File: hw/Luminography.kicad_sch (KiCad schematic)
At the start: 109 parts, among them J1 USB_C_Receptacle_PowerOnly_6P, J2 Conn_01x04, Q1 MMBT3904, Q2 2N7002, SW1 SW_Push, U1 LTC4054ES5-4.2, U10 MAX98357AETE+, U100 BH1750FVI-TR, U101 BH1750FVI-TR, U102 BH1750FVI-TR, U103 BH1750FVI-TR, U104 BH1750FVI-TR, U105 BH1750FVI-TR, U106 BH1750FVI-TR, U107 BH1750FVI-TR, U108 BH1750FVI-TR, U109 BH1750FVI-TR, U110 BH1750FVI-TR, U111 BH1750FVI-TR, U112 BH1750FVI-TR, U113 BH1750FVI-TR, U114 BH1750FVI-TR, U115 BH1750FVI-TR, U116 BH1750FVI-TR, U117 BH1750FVI-TR, U118 BH1750FVI-TR, U119 BH1750FVI-TR, U120 BH1750FVI-TR, U121 BH1750FVI-TR, U122 BH1750FVI-TR, U123 BH1750FVI-TR, U2 XS3A1T3157GMX, U3 SPX3819M5-L-3-3, U4 MAX17048G+T10, U5 STM32G030K6Tx, U6 ZJY128R-IG01, U7 W25Q16JVUXIQ, U8 BMI270, U9 MMC5603NJ, X1 12.288MHz

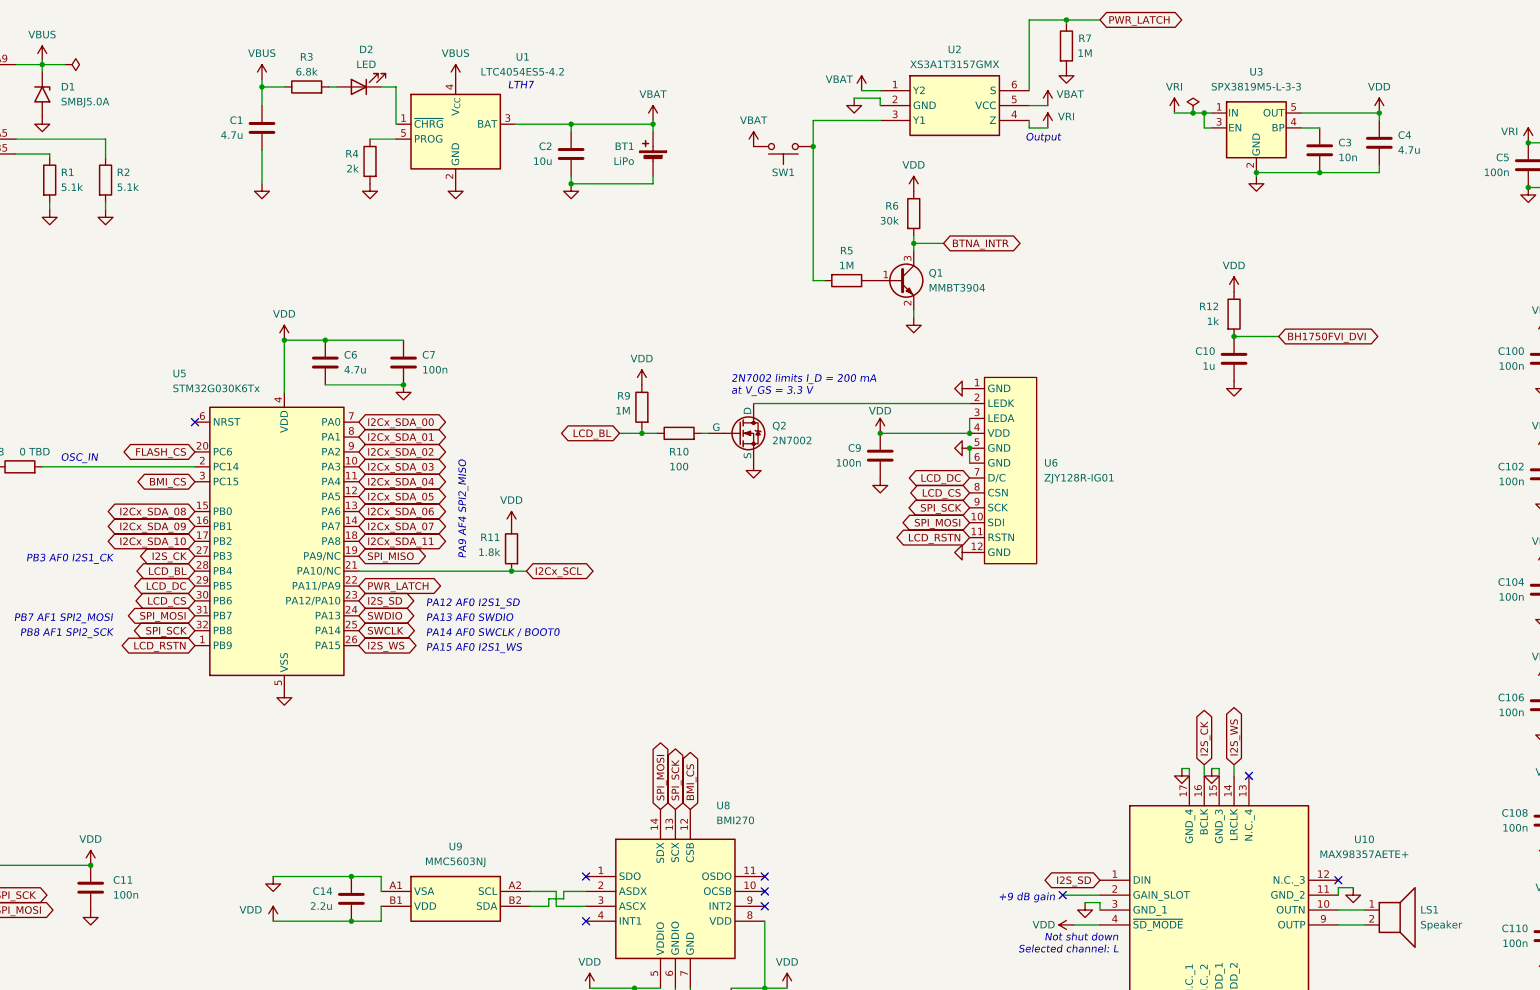
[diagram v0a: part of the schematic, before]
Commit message: 🚧 Routing WIP
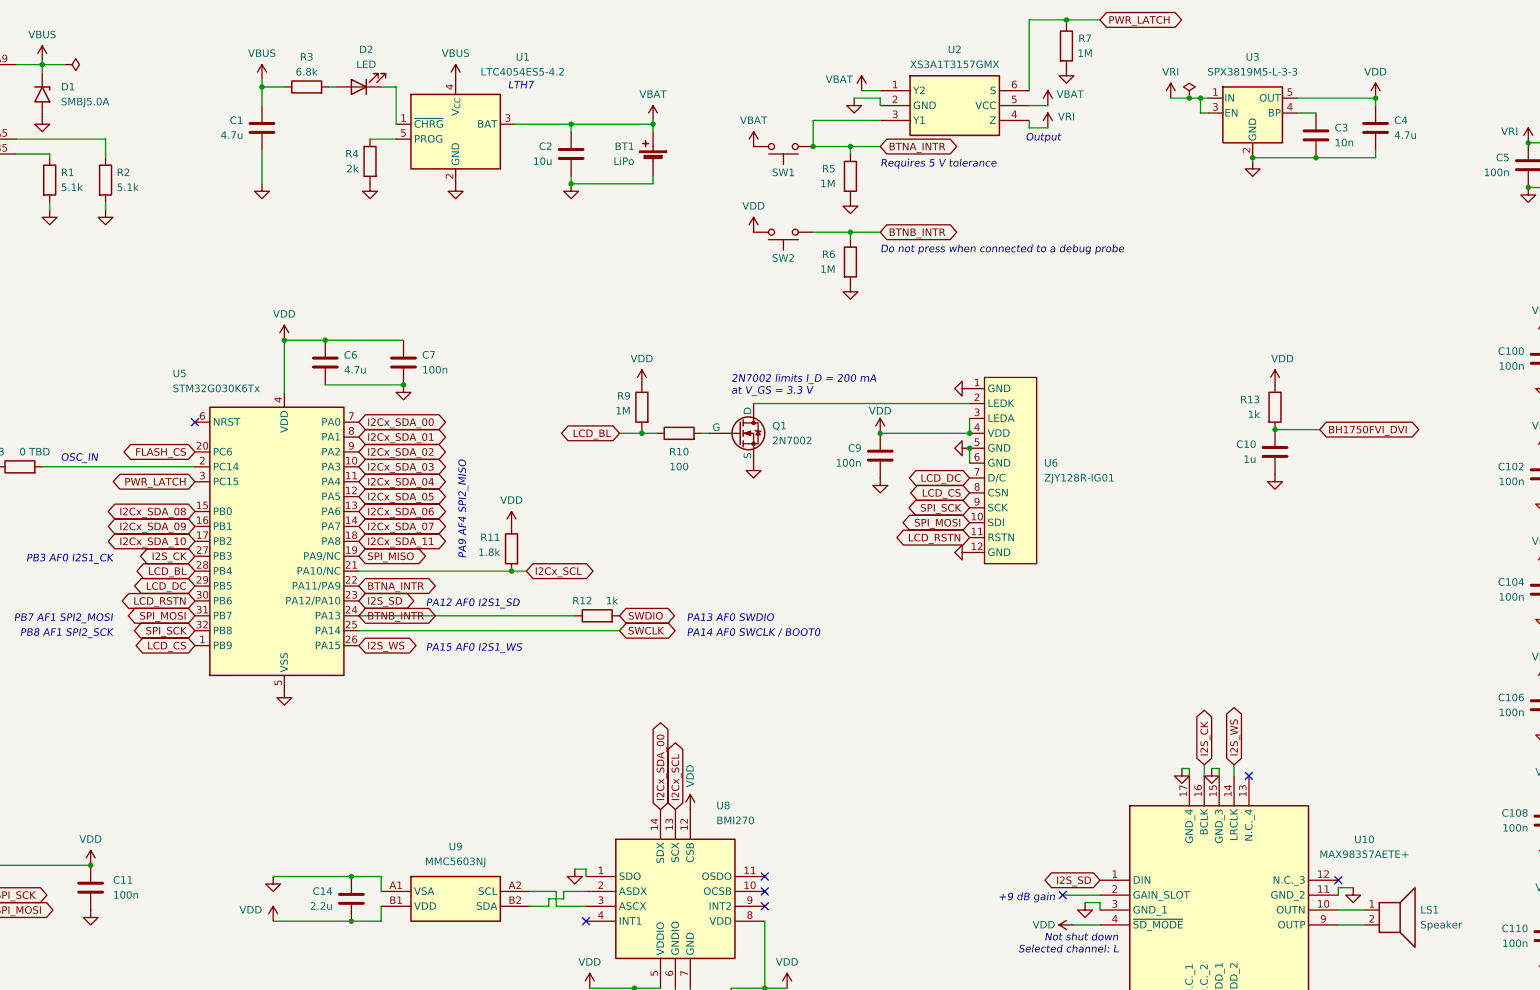
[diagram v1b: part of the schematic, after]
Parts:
- removed Q1: MMBT3904, Package_TO_SOT_SMD:SOT-23, symbol Transistor_BJT:MMBT3904
- removed R5: 1M, Resistor_SMD:R_0402_1005Metric, symbol Device:R
- added R12: 1k, Resistor_SMD:R_0402_1005Metric, symbol Device:R
- added R6: 1M, Resistor_SMD:R_0402_1005Metric, symbol Device:R
- added SW2: SW_Push, Button_Switch_SMD:SW_SPST_TL3342, symbol Switch:SW_Push
- R5: renamed from R6; value 30k -> 1M
- renumbered Q2 to Q1, R12 to R13
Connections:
- net BTNA_INTR: now also R5.1, SW1.2, U2.3 (Y1), U5.22 (PA11/PA9); no longer R5.2
- net GND: now also R5.2, U8.1 (SDO), R6.2
- net I2Cx_SCL: now also U8.13 (SCX)
- net I2Cx_SDA_00: now also U8.14 (SDX)
- net LCD_CS: now also U5.1 (PB9); no longer U5.30 (PB6)
- net LCD_RSTN: now also U5.30 (PB6); no longer U5.1 (PB9)
- net PWR_LATCH: now also U5.3 (PC15); no longer U5.22 (PA11/PA9)
- net SPI_MOSI: no longer U8.14 (SDX)
- net SPI_SCK: no longer U8.13 (SCX)
- net SWDIO: now also R12.2; no longer U5.24 (PA13)
- net VDD: now also U8.12 (CSB), SW2.1; no longer R5.1
- removed net BMI_CS: U5.3 (PC15), U8.12 (CSB)
- new net BTNB_INTR: R12.1, R6.1, SW2.2, U5.24 (PA13)
- no-connect marks 16 -> 15
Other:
- note added: "Do not press when connected to a debug probe"
- note added: "Requires 5 V tolerance"
- moved on the sheet: C10, C3, C4, R13, R5, U3

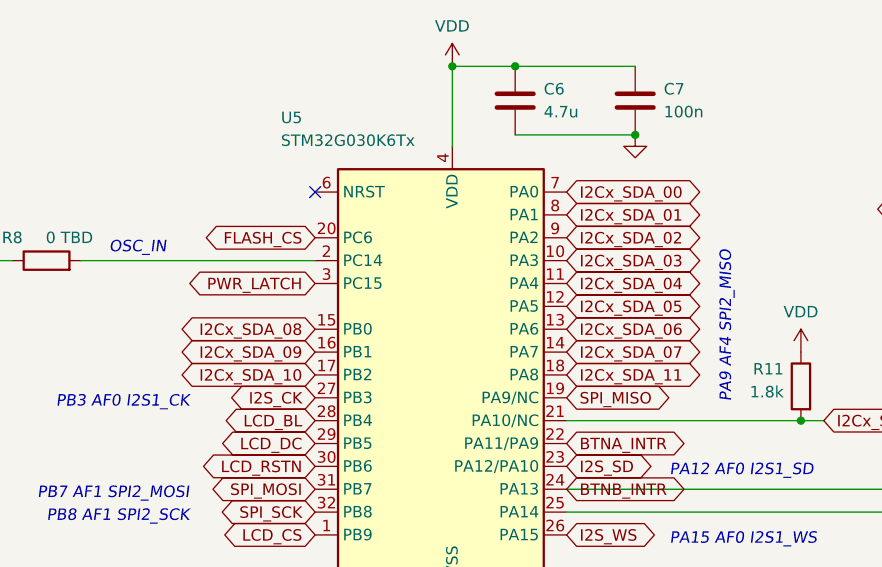
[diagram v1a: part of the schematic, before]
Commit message: Board design almost done, do later
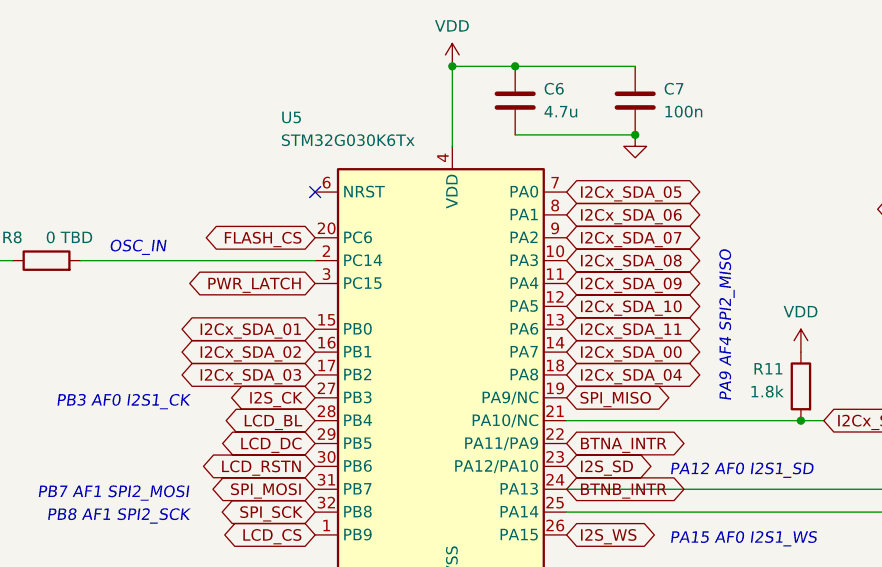
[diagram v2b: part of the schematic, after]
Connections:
- net I2Cx_SDA_00: now also U5.14 (PA7); no longer U5.7 (PA0)
- net I2Cx_SDA_01: now also U5.15 (PB0); no longer U5.8 (PA1)
- net I2Cx_SDA_02: now also U5.16 (PB1); no longer U5.9 (PA2)
- net I2Cx_SDA_03: now also U5.17 (PB2); no longer U5.10 (PA3)
- net I2Cx_SDA_04: now also U5.18 (PA8); no longer U5.11 (PA4)
- net I2Cx_SDA_05: now also U5.7 (PA0); no longer U5.12 (PA5)
- net I2Cx_SDA_06: now also U5.8 (PA1); no longer U5.13 (PA6)
- net I2Cx_SDA_07: now also U5.9 (PA2); no longer U5.14 (PA7)
- net I2Cx_SDA_08: now also U5.10 (PA3); no longer U5.15 (PB0)
- net I2Cx_SDA_09: now also U5.11 (PA4); no longer U5.16 (PB1)
- net I2Cx_SDA_10: now also U5.12 (PA5); no longer U5.17 (PB2)
- net I2Cx_SDA_11: now also U5.13 (PA6); no longer U5.18 (PA8)
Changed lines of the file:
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@@
     )
   )
-  (global_label "I2Cx_SDA_02" (shape bidirectional) (at 100.33 88.9 0) (fields_autoplaced)
+  (global_label "I2Cx_SDA_07" (shape bidirectional) (at 100.33 88.9 0) (fields_autoplaced)
     (effects (font (size 1.27 1.27)) (justify left))
     (property "Intersheetrefs" "${INTERSHEET_REFS}" (at 116.4612 88.9 0)
@@
     )
   )
-  (global_label "I2Cx_SDA_07" (shape bidirectional) (at 100.33 101.6 0) (fields_autoplaced)
+  (global_label "I2Cx_SDA_00" (shape bidirectional) (at 100.33 101.6 0) (fields_autoplaced)
     (effects (font (size 1.27 1.27)) (justify left))
     (property "Intersheetrefs" "${INTERSHEET_REFS}" (at 116.4612 101.6 0)
@@
     )
   )
-  (global_label "I2Cx_SDA_03" (shape bidirectional) (at 100.33 91.44 0) (fields_autoplaced)
+  (global_label "I2Cx_SDA_08" (shape bidirectional) (at 100.33 91.44 0) (fields_autoplaced)
     (effects (font (size 1.27 1.27)) (justify left))
     (property "Intersheetrefs" "${INTERSHEET_REFS}" (at 116.4612 91.44 0)
@@
     )
   )
-  (global_label "I2Cx_SDA_08" (shape bidirectional) (at 72.39 99.06 180) (fields_autoplaced)
+  (global_label "I2Cx_SDA_01" (shape bidirectional) (at 72.39 99.06 180) (fields_autoplaced)
     (effects (font (size 1.27 1.27)) (justify right))
     (property "Intersheetrefs" "${INTERSHEET_REFS}" (at 56.2588 99.06 0)
@@
     )
   )
-  (global_label "I2Cx_SDA_10" (shape bidirectional) (at 72.39 104.14 180) (fields_autoplaced)
+  (global_label "I2Cx_SDA_03" (shape bidirectional) (at 72.39 104.14 180) (fields_autoplaced)
     (effects (font (size 1.27 1.27)) (justify right))
     (property "Intersheetrefs" "${INTERSHEET_REFS}" (at 56.2588 104.14 0)
@@
     )
   )
-  (global_label "I2Cx_SDA_04" (shape bidirectional) (at 100.33 93.98 0) (fields_autoplaced)
+  (global_label "I2Cx_SDA_09" (shape bidirectional) (at 100.33 93.98 0) (fields_autoplaced)
     (effects (font (size 1.27 1.27)) (justify left))
     (property "Intersheetrefs" "${INTERSHEET_REFS}" (at 116.4612 93.98 0)
@@
     )
   )
-  (global_label "I2Cx_SDA_01" (shape bidirectional) (at 100.33 86.36 0) (fields_autoplaced)
+  (global_label "I2Cx_SDA_06" (shape bidirectional) (at 100.33 86.36 0) (fields_autoplaced)
     (effects (font (size 1.27 1.27)) (justify left))
     (property "Intersheetrefs" "${INTERSHEET_REFS}" (at 116.4612 86.36 0)
@@
     )
   )
-  (global_label "I2Cx_SDA_11" (shape bidirectional) (at 100.33 104.14 0) (fields_autoplaced)
+  (global_label "I2Cx_SDA_04" (shape bidirectional) (at 100.33 104.14 0) (fields_autoplaced)
     (effects (font (size 1.27 1.27)) (justify left))
     (property "Intersheetrefs" "${INTERSHEET_REFS}" (at 116.4612 104.14 0)
@@
     )
   )
-  (global_label "I2Cx_SDA_00" (shape bidirectional) (at 100.33 83.82 0) (fields_autoplaced)
+  (global_label "I2Cx_SDA_05" (shape bidirectional) (at 100.33 83.82 0) (fields_autoplaced)
     (effects (font (size 1.27 1.27)) (justify left))
     (property "Intersheetrefs" "${INTERSHEET_REFS}" (at 116.4612 83.82 0)
@@
     )
   )
-  (global_label "I2Cx_SDA_09" (shape bidirectional) (at 72.39 101.6 180) (fields_autoplaced)
+  (global_label "I2Cx_SDA_02" (shape bidirectional) (at 72.39 101.6 180) (fields_autoplaced)
     (effects (font (size 1.27 1.27)) (justify right))
     (property "Intersheetrefs" "${INTERSHEET_REFS}" (at 56.2588 101.6 0)
@@
     )
   )
-  (global_label "I2Cx_SDA_06" (shape bidirectional) (at 100.33 99.06 0) (fields_autoplaced)
+  (global_label "I2Cx_SDA_11" (shape bidirectional) (at 100.33 99.06 0) (fields_autoplaced)
     (effects (font (size 1.27 1.27)) (justify left))
     (property "Intersheetrefs" "${INTERSHEET_REFS}" (at 116.4612 99.06 0)
@@
     )
   )
-  (global_label "I2Cx_SDA_05" (shape bidirectional) (at 100.33 96.52 0) (fields_autoplaced)
+  (global_label "I2Cx_SDA_10" (shape bidirectional) (at 100.33 96.52 0) (fields_autoplaced)
     (effects (font (size 1.27 1.27)) (justify left))
     (property "Intersheetrefs" "${INTERSHEET_REFS}" (at 116.4612 96.52 0)

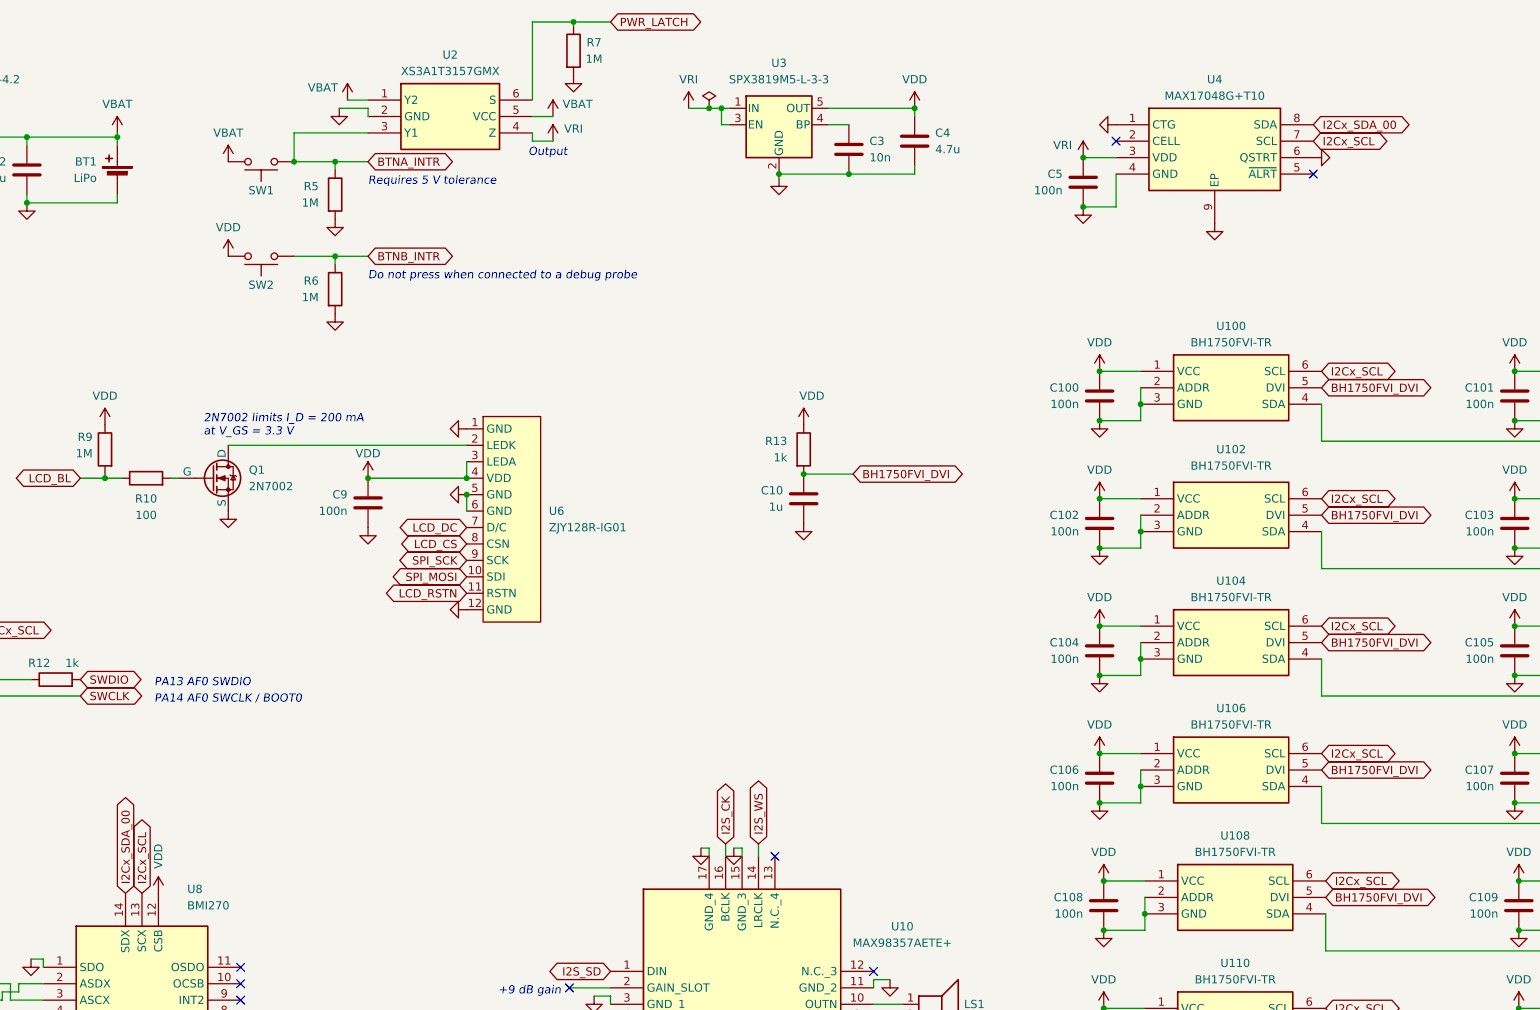
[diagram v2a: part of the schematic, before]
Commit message: Finish routing
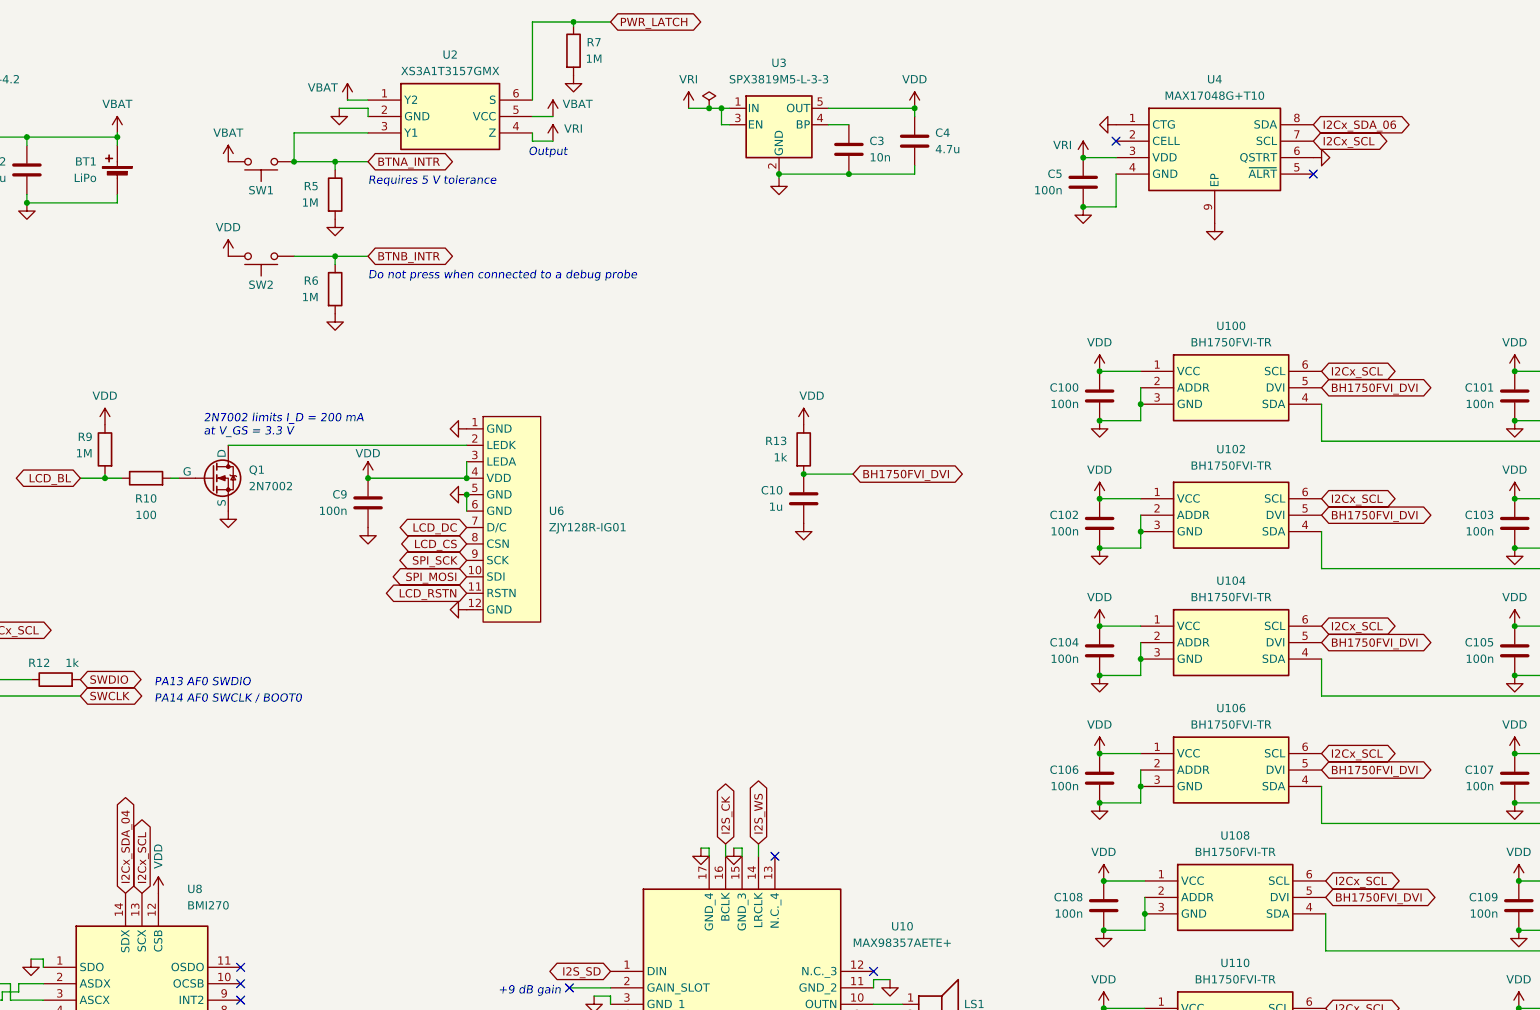
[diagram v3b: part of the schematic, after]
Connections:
- net I2Cx_SDA_00: no longer U4.8 (SDA), U8.14 (SDX)
- net I2Cx_SDA_04: now also U8.14 (SDX)
- net I2Cx_SDA_06: now also U4.8 (SDA)
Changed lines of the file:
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@@
     )
   )
-  (global_label "I2Cx_SDA_00" (shape bidirectional) (at 335.28 31.115 0) (fields_autoplaced)
+  (global_label "I2Cx_SDA_06" (shape bidirectional) (at 335.28 31.115 0) (fields_autoplaced)
     (effects (font (size 1.27 1.27)) (justify left))
     (property "Intersheetrefs" "${INTERSHEET_REFS}" (at 351.4112 31.115 0)
@@
     )
   )
-  (global_label "I2Cx_SDA_00" (shape bidirectional) (at 151.765 149.86 90) (fields_autoplaced)
+  (global_label "I2Cx_SDA_04" (shape bidirectional) (at 151.765 149.86 90) (fields_autoplaced)
     (effects (font (size 1.27 1.27)) (justify left))
     (property "Intersheetrefs" "${INTERSHEET_REFS}" (at 151.765 133.7288 90)
